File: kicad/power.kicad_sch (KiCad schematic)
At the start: 63 parts, among them J9 USB_C_Receptacle_USB2.0_16P, SW15 PH_IND, T1 475uH, U20 TPS7A39, U21 SN6505BDBV, U22 TPS2116DRL, U23 TPS62172DSG, U25 TPS7A2009, U26 TPS62171DSG, U27 TPS7A4101, U28 TPS61391, U29 CH224K

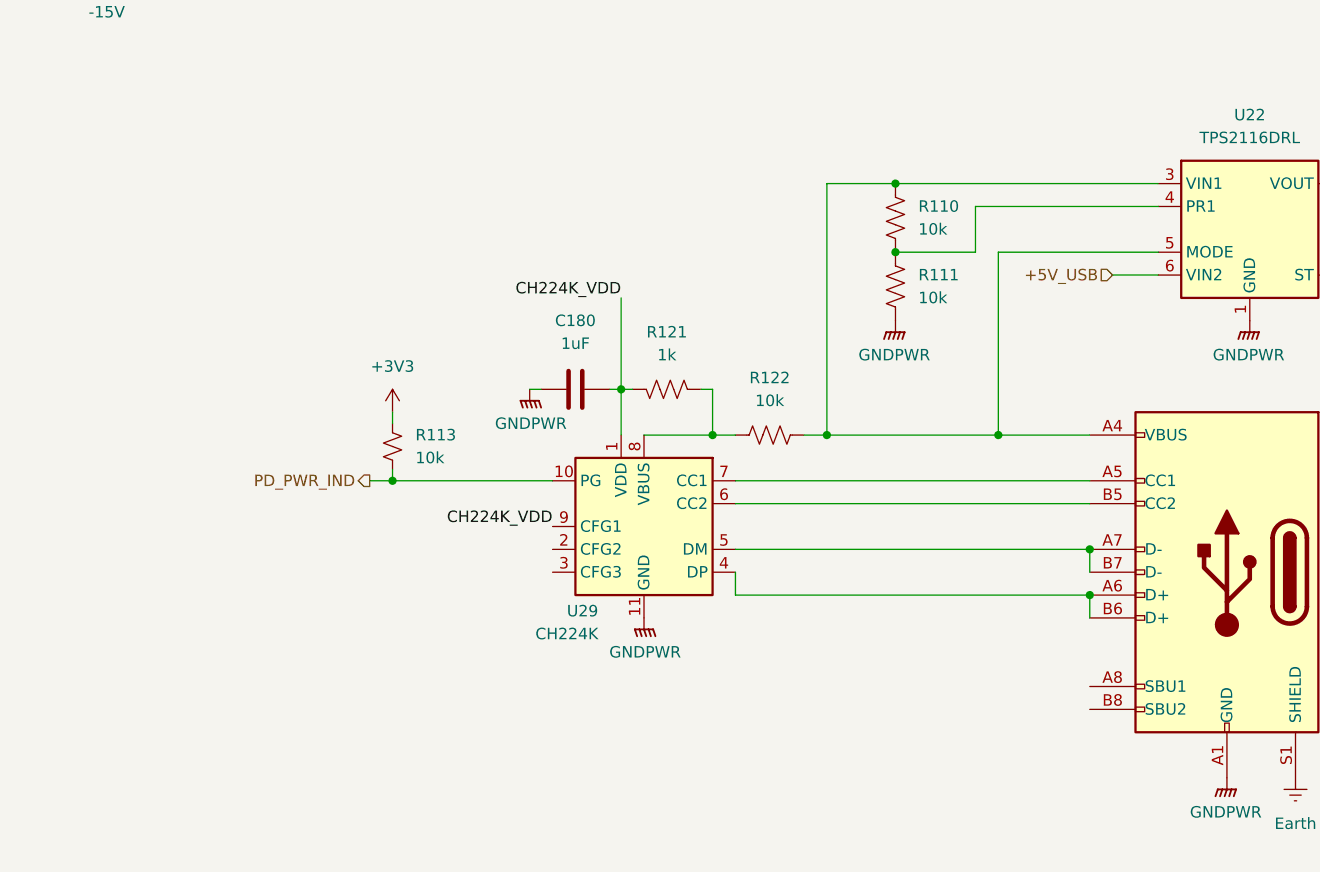
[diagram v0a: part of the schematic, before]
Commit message: bypass caps
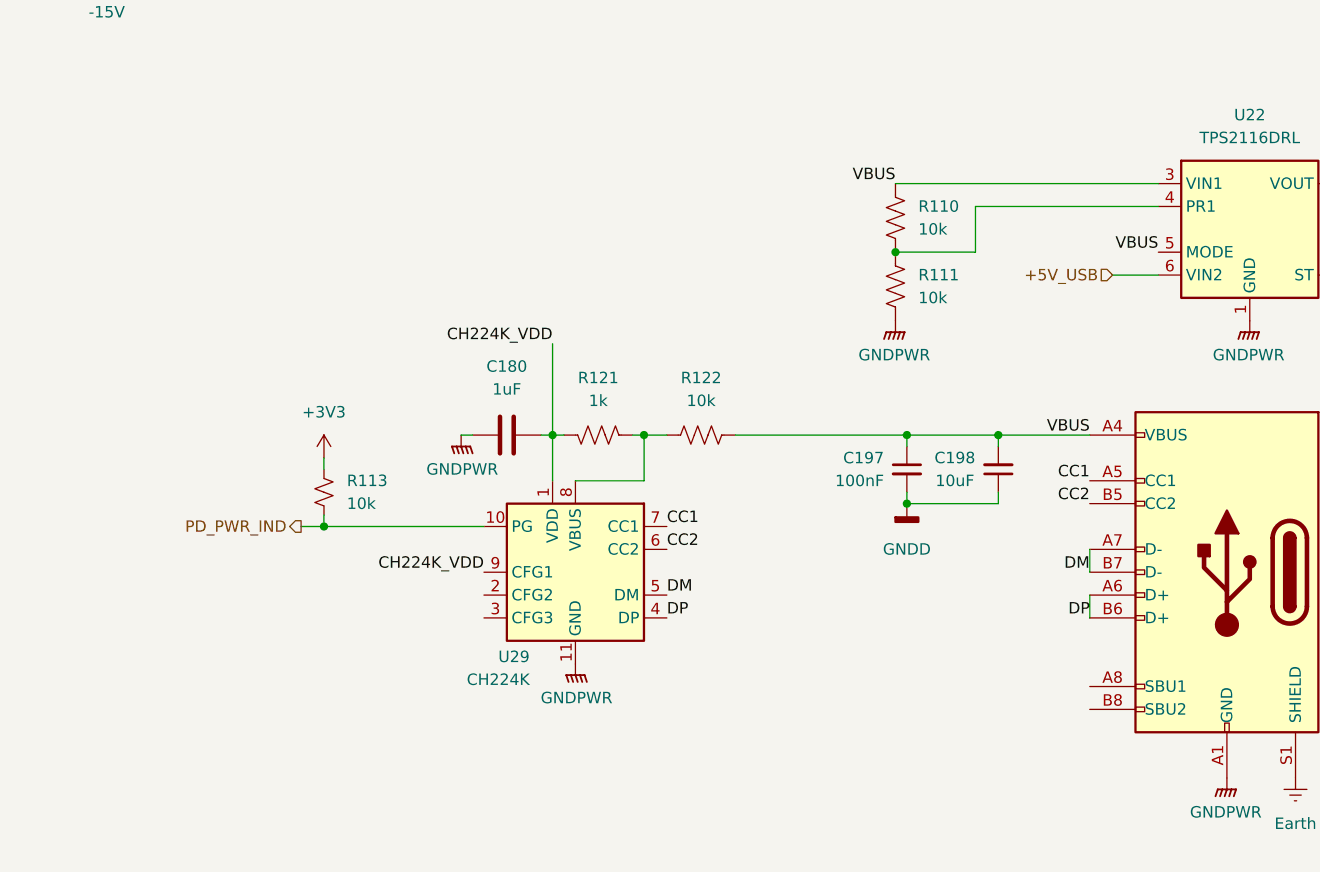
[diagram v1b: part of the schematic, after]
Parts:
- added C197: 100nF, symbol Device:C_Small
- added C198: 10uF, symbol Device:C_Small
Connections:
- net GND1: now also C197.2, C198.1
- net VBUS: now reaches J9.A4 (VBUS), J9.A9 (VBUS), J9.B4 (VBUS), J9.B9 (VBUS), R110.1, R122.2, U22.3 (VIN1), U22.5 (MODE)
- net VBUS: now also C197.1, C198.2
- net CC1: now reaches J9.A5 (CC1), U29.7 (CC1)
- net DP: now reaches J9.A6 (D+), J9.B6 (D+), U29.4 (DP)
- net DM: now reaches J9.A7 (D-), J9.B7 (D-), U29.5 (DM)
- net CC2: now reaches J9.B5 (CC2), U29.6 (CC2)
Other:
- moved on the sheet: C180, R113, R121, R122, U29
